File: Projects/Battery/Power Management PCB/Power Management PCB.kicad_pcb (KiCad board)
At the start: 2 copper layers, 62 x 29 mm, 19 parts, among them J1 Conn_01x02_Pin, J2 Conn_01x02_Pin, J3 Conn_01x02_Pin, J4 Conn_01x02_Pin, U1 LM317_SOT-223, U2 LM317_SOT-223, U3 LM317_SOT-223

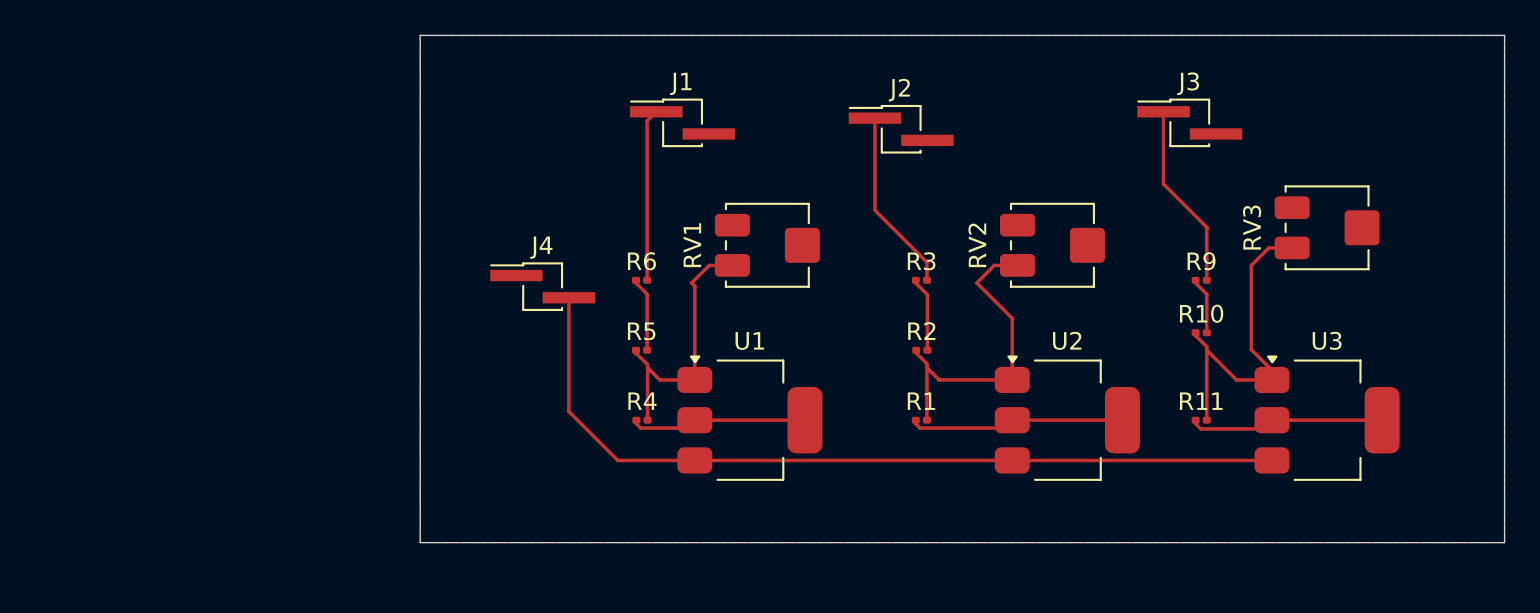
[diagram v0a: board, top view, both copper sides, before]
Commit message: 9/22 pcb
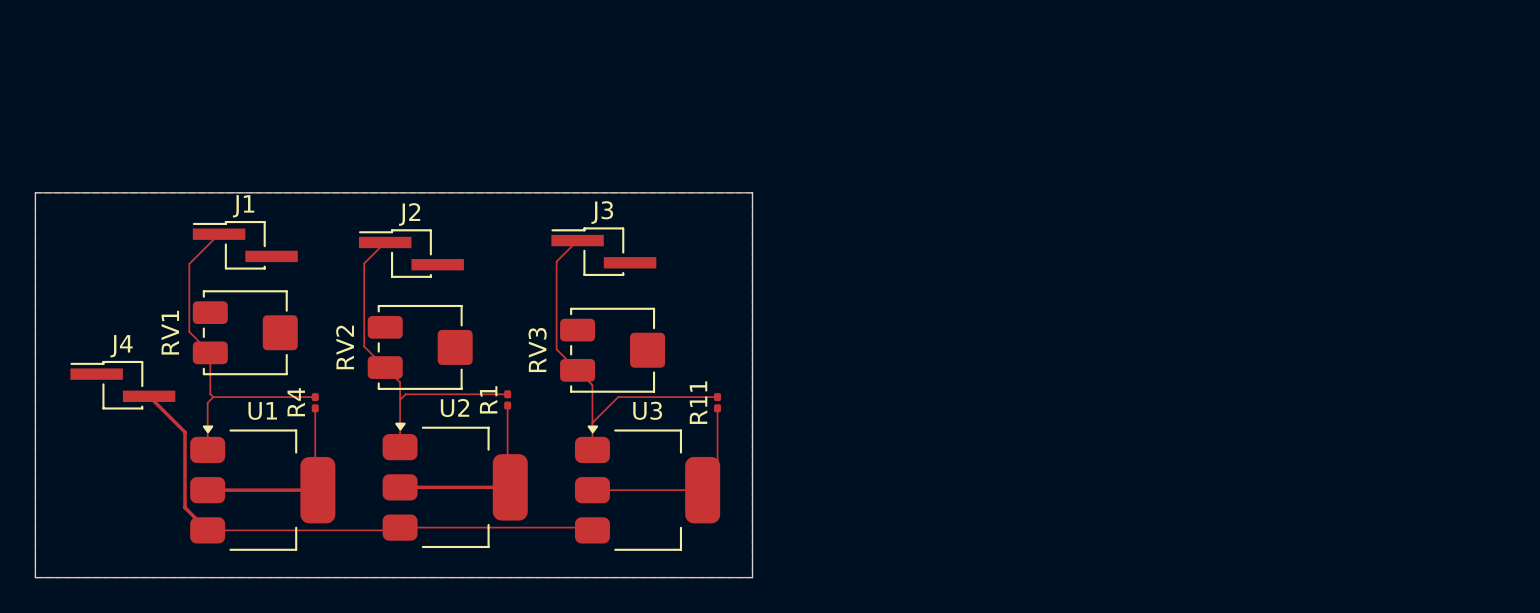
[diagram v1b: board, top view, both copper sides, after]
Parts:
- removed R10, R2, R5: 1,000, Resistor_SMD:R_0201_0603Metric
- removed R3, R6, R9: 10,000, Resistor_SMD:R_0201_0603Metric
- R4: value 300 -> 125
- moved RV3 41.4 mm to (150.0, 112.0)
- moved U3 39.1 mm to (152.0, 120.0)
- moved RV2 36.6 mm to (139.0, 111.8)
- moved U2 35.2 mm to (141.0, 119.8)
- moved J3 34.3 mm to (149.5, 106.4)
- moved RV1 30.3 mm to (129.0, 111.0)
- moved J2 28.9 mm to (138.5, 106.5)
- moved U1 28.1 mm to (130.0, 120.0)
- moved R11 27.7 mm to (156.0, 115.0), turned to 90 degrees
- moved J1 26.0 mm to (129.0, 106.0)
- moved J4 24.7 mm to (122.0, 114.0)
- moved R1 23.7 mm to (144.0, 114.8), turned to 90 degrees
- moved R4 18.7 mm to (133.0, 115.0), turned to 90 degrees
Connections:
- R1 pad 2: Net-(U2-ADJ) -> Net-(J2-Pin_1)
- R11 pad 2: Net-(U3-ADJ) -> Net-(J3-Pin_1)
- R4 pad 2: Net-(U1-ADJ) -> Net-(J1-Pin_1)
- RV1 pad 1: Net-(U1-ADJ) -> Net-(J1-Pin_1)
- RV2 pad 1: Net-(U2-ADJ) -> Net-(J2-Pin_1)
- RV3 pad 1: Net-(U3-ADJ) -> Net-(J3-Pin_1)
- U1 pad 1: Net-(U1-ADJ) -> Net-(J1-Pin_1)
- U2 pad 1: Net-(U2-ADJ) -> Net-(J2-Pin_1)
- U3 pad 1: Net-(U3-ADJ) -> Net-(J3-Pin_1)
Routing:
- net Net-(U3-ADJ): track 19.7 -> 0.00 mm
- net Net-(U2-ADJ): track 18.5 -> 0.00 mm
- net Net-(J4-Pin_2): track 47.9 -> 31.2 mm
- net Net-(U1-ADJ): track 15.8 -> 0.00 mm
- net Net-(J3-Pin_1): track 10.7 -> 21.1 mm
- net Net-(J1-Pin_1): track 9.85 -> 19.6 mm
- net Net-(J2-Pin_1): track 10.5 -> 19.7 mm
- net Net-(R2-Pad2): track 4.28 -> 0.00 mm
- net Net-(R5-Pad2): track 4.27 -> 0.00 mm
- net Net-(R10-Pad2): track 3.27 -> 0.00 mm
- net Net-(U2-VO): track 13.0 -> 11.0 mm
- net Net-(U1-VO): track 10.8 -> 11.9 mm
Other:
- board size 62 x 29 mm -> 41 x 22 mm
